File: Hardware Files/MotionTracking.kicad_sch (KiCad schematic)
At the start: 28 parts, among them J1 Micro_SD_Card_Det1, J2 USB_B_Micro, U1 LSM6DSV16XTR, U2 ADP2302ARDZ-3.3, U4 STM32F411RET6, Y1 16MHz

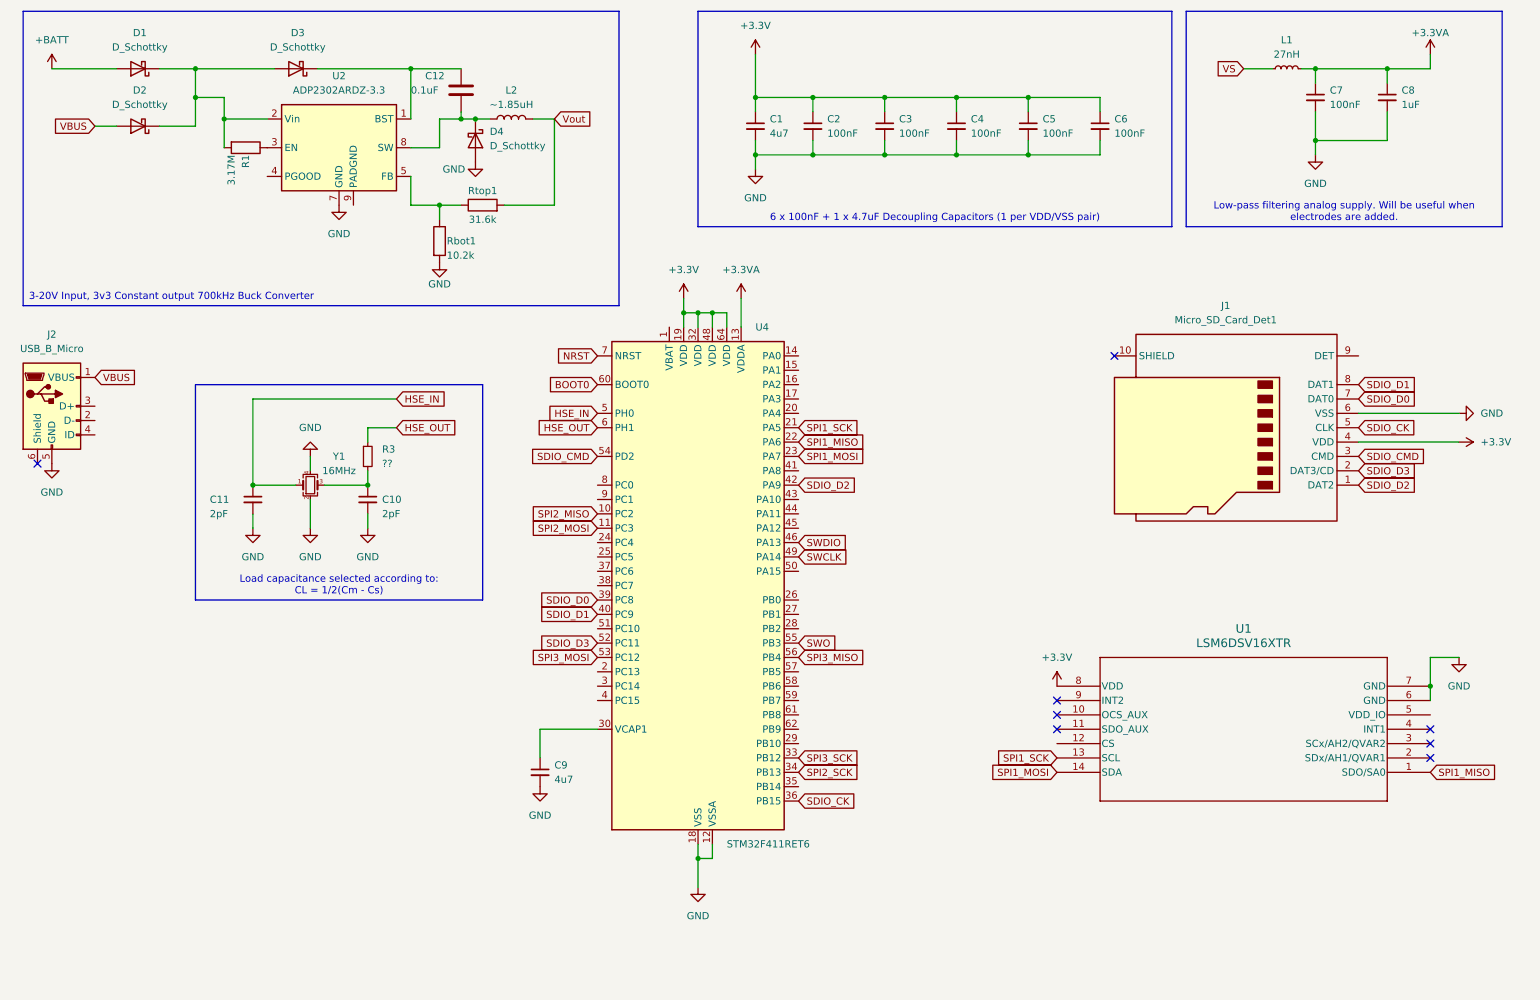
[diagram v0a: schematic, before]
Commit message: Actually changed pins this time
did not save before pushing
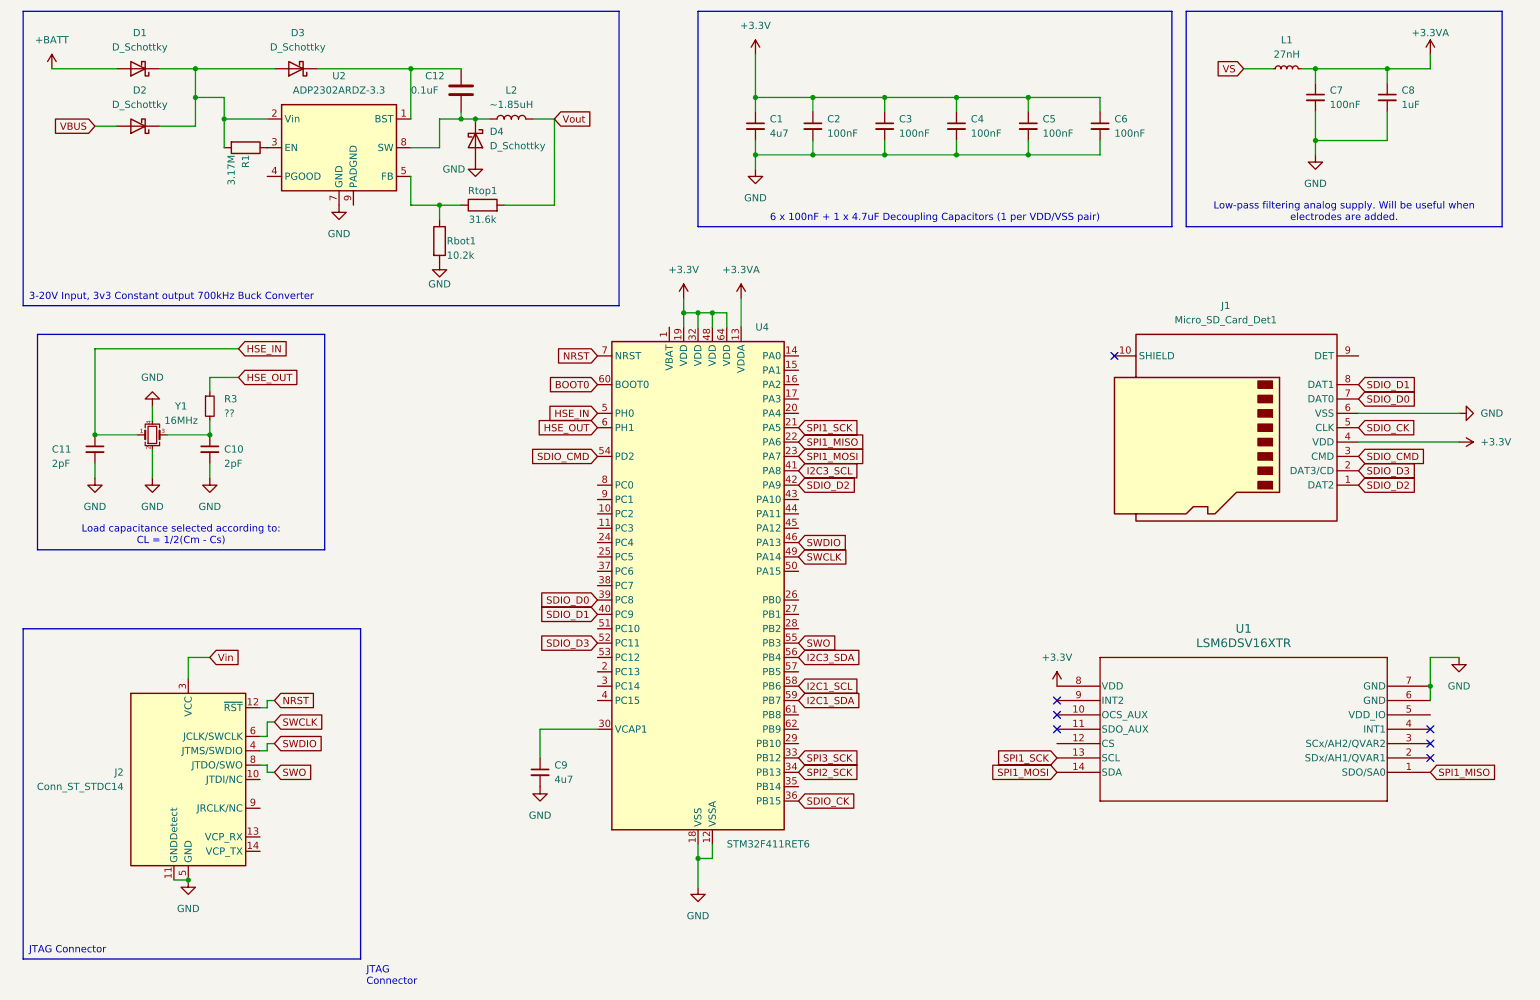
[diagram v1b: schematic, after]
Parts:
- removed J2: USB_B_Micro, symbol Connector:USB_B_Micro
- added J2: Conn_ST_STDC14, symbol Connector:Conn_ST_STDC14
- C1, C10, C11, C12, C2, C3, C4, C5, C6, C7, C8, C9: footprint Capacitor_SMD:C_0603_1608Metric_Pad1.08x0.95mm_HandSolder -> (none)
- D1, D2, D3, D4: footprint Diode_SMD:D_SOD-323 -> (none)
- L1, L2: footprint Inductor_SMD:L_0603_1608Metric_Pad1.05x0.95mm_HandSolder -> (none)
- R1, R3, Rbot1, Rtop1: footprint Resistor_SMD:R_0603_1608Metric_Pad0.98x0.95mm_HandSolder -> (none)
- Y1: footprint Crystal:Crystal_SMD_SeikoEpson_TSX3225-4Pin_3.2x2.5mm_HandSoldering -> (none)
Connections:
- net GND: now also J2.11 (GNDDetect), J2.5 (GND), J2.7 (GND)
- net NRST: now also J2.12 (~{RST})
- net SWCLK: now also J2.6 (JCLK/SWCLK)
- net SWDIO: now also J2.4 (JTMS/SWDIO)
- net SWO: now also J2.8 (JTDO/SWO)
- net I2C3_SCL: now reaches U4.41 (PA8)
- net I2C1_SCL: now reaches U4.58 (PB6)
- net I2C1_SDA: now reaches U4.59 (PB7)
- net SPI2_MISO: no longer names the net of U4.10 (PC2)
- net SPI2_MOSI: no longer names the net of U4.11 (PC3)
- net SPI3_MISO renamed I2C3_SDA
- net SPI3_MOSI: no longer names the net of U4.53 (PC12)
- new net Vin: J2.3 (VCC)
- no-connect marks 8 -> 7
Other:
- moved on the sheet: C10, C11, R3, Y1
